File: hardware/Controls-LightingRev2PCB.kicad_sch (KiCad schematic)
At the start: 31 parts, among them IC3 ACS724LLCTR-05AU-T, IC4 ACS724LLCTR-05AU-T, IC5 TLV70433DBVT, IC6 ACS724LLCTR-05AU-T, J1 53307-2471, J2 MX150_02x08_RightAngle, J3 53307-2471, Q3 IRLML0030, Q5 IRLML0030, U5 SN74LV1T34DBV

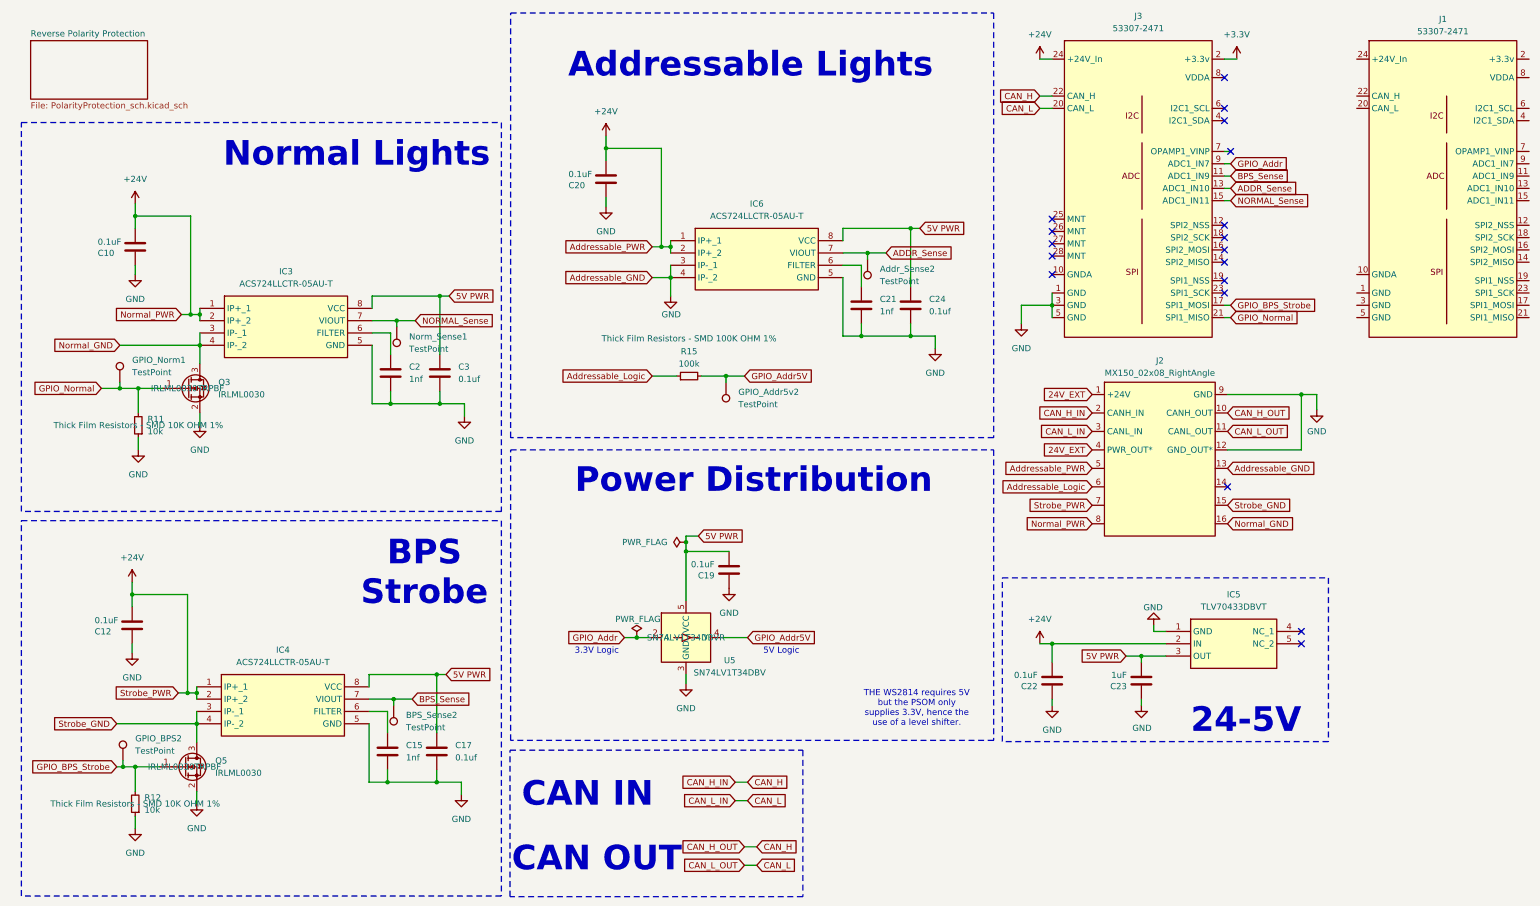
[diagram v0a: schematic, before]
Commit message: Rev B schematic Review with new IC
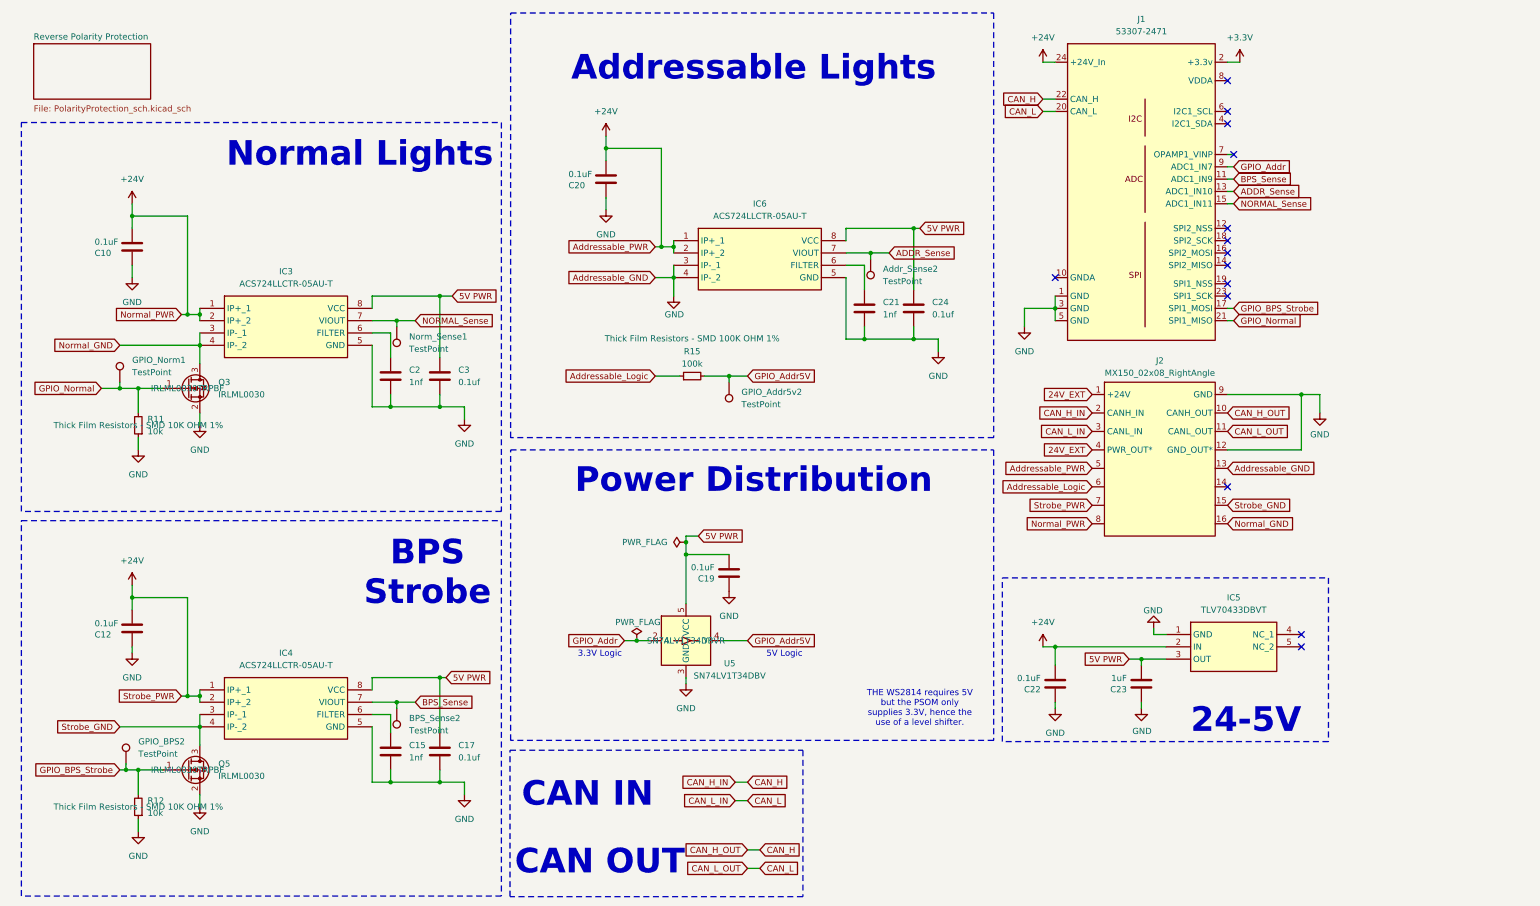
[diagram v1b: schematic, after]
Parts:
- removed J3: 53307-2471, UTSVT_Connectors:PeripheralSOM, symbol utsvt-connectors:PeripheralSOMConnector
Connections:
- net +24V: now also J1.24 (+24V_In)
- net +3.3V: now also J1.2 (+3.3v)
- net ADDR_Sense: now also J1.13 (ADC1_IN10)
- net BPS_Sense: now also J1.11 (ADC1_IN9)
- net CAN_H: now also J1.22 (CAN_H)
- net CAN_L: now also J1.20 (CAN_L)
- net GND: now also J1.1 (GND), J1.3 (GND), J1.5 (GND)
- net GPIO_Addr: now also J1.9 (ADC1_IN7)
- net GPIO_BPS_Strobe: now also J1.17 (SPI1_MOSI)
- net GPIO_Normal: now also J1.21 (SPI1_MISO)
- net NORMAL_Sense: now also J1.15 (ADC1_IN11)
- no-connect marks 18 -> 14
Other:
- moved on the sheet: Addr_Sense2, BPS_Sense2, C10, C12, C15, C17, C19, C2, C21, C22, C23, C24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
